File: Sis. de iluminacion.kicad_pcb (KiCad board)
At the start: 2 copper layers, 48 parts, among them J1 Screw_Terminal_01x02, J2 Screw_Terminal_01x04, J3 Screw_Terminal_01x02, J5 Screw_Terminal_01x02, J7 Screw_Terminal_01x02, J9 Screw_Terminal_01x02, K10 Relay_DPDT, K11 Relay_DPDT, K8 Relay_DPDT, K9 Relay_DPDT, Q4 BC547, Q5 BC547, Q6 BC547, Q7 BC547, U1 ESP32_DEVKITC, U10 PC817, U11 PC817, U12 PC817, U13 PC817, U3 L7805

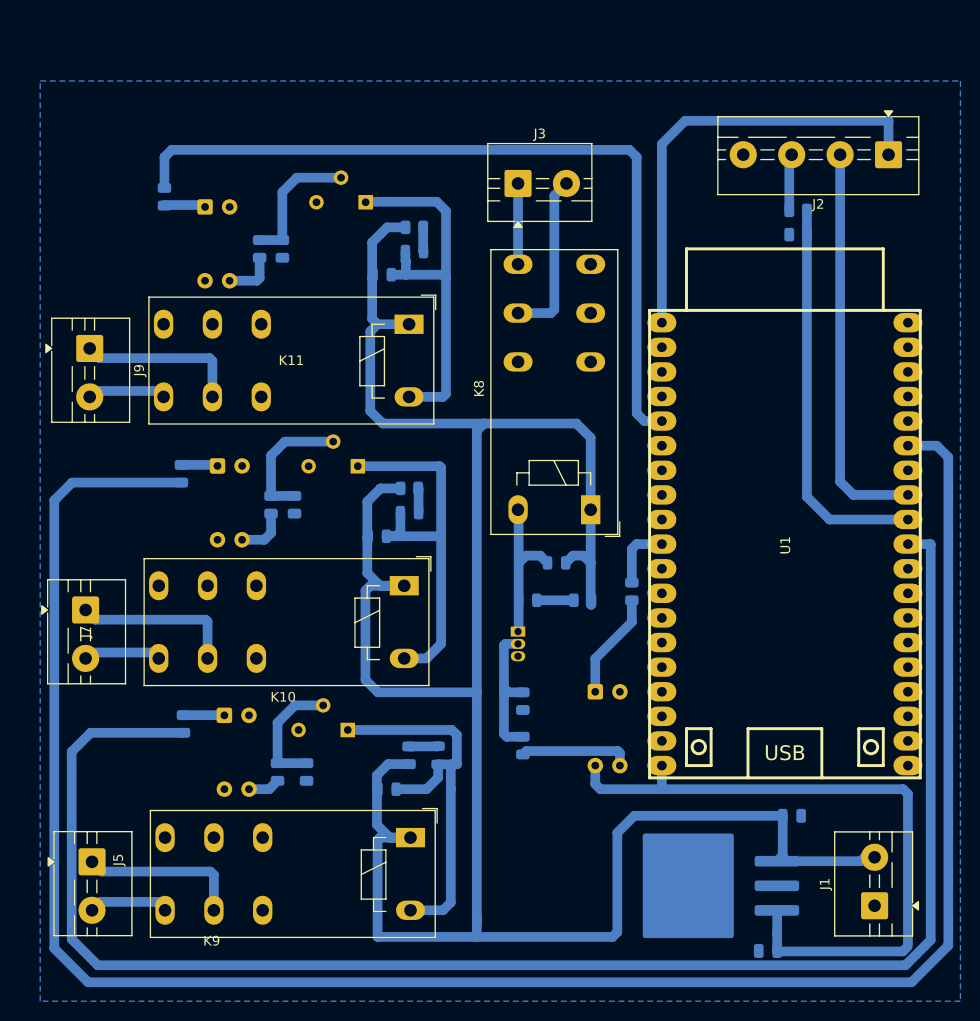
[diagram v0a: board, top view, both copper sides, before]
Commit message: Rele wifi
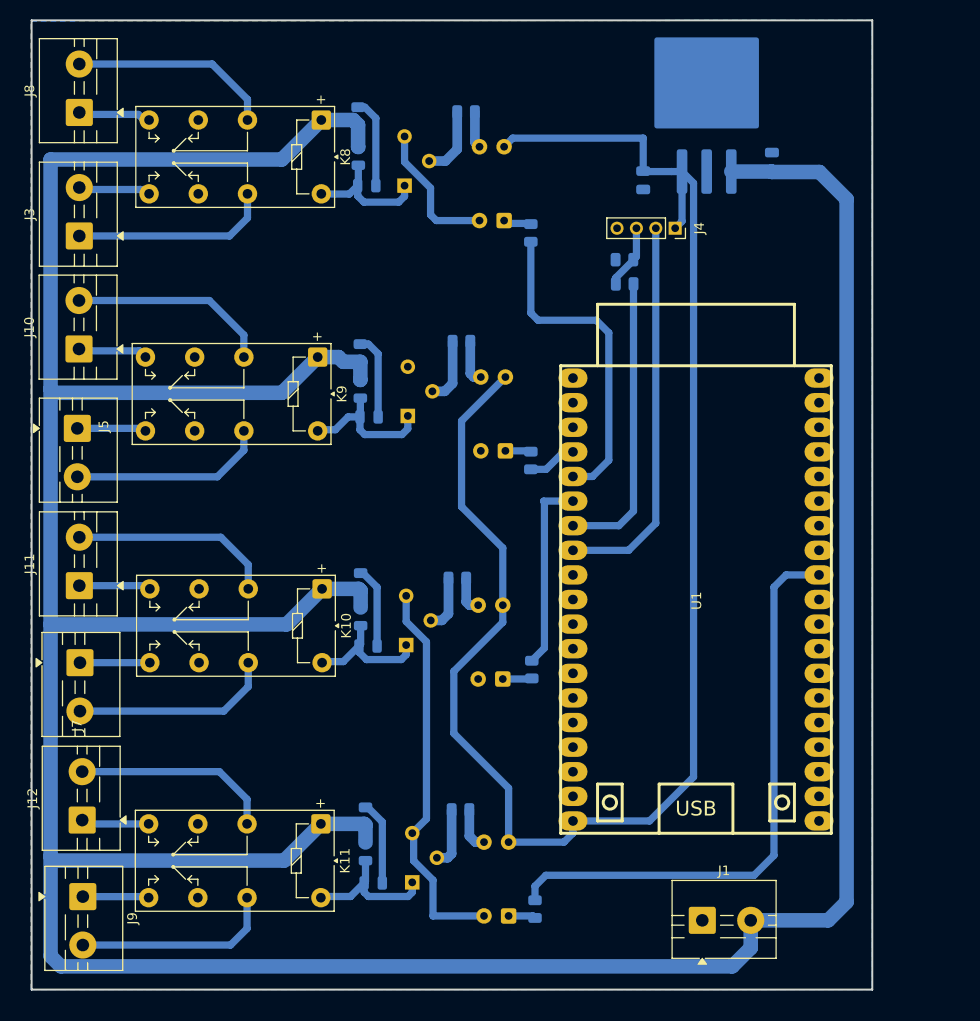
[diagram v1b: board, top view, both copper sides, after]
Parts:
- removed J2: Screw_Terminal_01x04, TerminalBlock:TerminalBlock_MaiXu_MX126-5.0-04P_1x04_P5.00mm
- removed R26, R31, R35, R39: 10K, Resistor_SMD:R_0805_2012Metric
- added J10: Screw_Terminal_01x02, TerminalBlock:TerminalBlock_MaiXu_MX126-5.0-02P_1x02_P5.00mm, F.Cu at (185.0, 74.2)
- added J11: Screw_Terminal_01x02, TerminalBlock:TerminalBlock_MaiXu_MX126-5.0-02P_1x02_P5.00mm, F.Cu at (185.0, 98.6)
- added J12: Screw_Terminal_01x02, TerminalBlock:TerminalBlock_MaiXu_MX126-5.0-02P_1x02_P5.00mm, F.Cu at (185.3, 122.8)
- added J4: Conn_01x04, Connector_PinSocket_2.00mm:PinSocket_1x04_P2.00mm_Vertical, F.Cu at (246.6, 61.7)
- added J8: Screw_Terminal_01x02, TerminalBlock:TerminalBlock_MaiXu_MX126-5.0-02P_1x02_P5.00mm, F.Cu at (185.0, 49.8)
- K10, K11, K8, K9: footprint Relay_THT:Relay_DPDT_Schrack-RT2-FormC_RM5mm -> Relay_THT:Relay_DPDT_Omron_G6A
- Q4: footprint Package_TO_SOT_THT:TO-92_Inline -> Package_TO_SOT_THT:TO-92_Wide
- R24, R28, R32, R36: value 1K -> 220
- moved R36 82.9 mm to (232.1, 132.0)
- moved U3 81.4 mm to (249.8, 48.2), turned to 90 degrees
- moved C2 80.6 mm to (243.2, 56.8), turned to -90 degrees
- moved U13 79.6 mm to (229.4, 132.7), turned to 90 degrees
- moved Q7 70.4 mm to (219.4, 129.2), turned to 90 degrees
- moved C1 67.6 mm to (256.5, 54.8), turned to 90 degrees
- moved R25 65.7 mm to (225.0, 49.7), turned to 180 degrees
- moved D21 65.3 mm to (215.4, 129.3)
- moved R37 61.5 mm to (224.4, 121.8), turned to 180 degrees
- moved R38 61.0 mm to (214.6, 122.4), turned to -90 degrees
- moved D22 59.6 mm to (214.6, 126.1), turned to -90 degrees
- moved J9 56.6 mm to (185.4, 130.7)
- moved R27 55.1 mm to (213.8, 50.1), turned to -90 degrees
- moved K11 52.4 mm to (210.0, 123.2), turned to -90 degrees
- moved K9 50.5 mm to (209.6, 75.0), turned to -90 degrees
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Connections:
- J3 pad 1: LED + -> 5V1
- J3 pad 2: 5V -> LED +
- J5 pad 1: V1 -> NO1
- J5 pad 2: NO1 -> V1
- J7 pad 1: V2 -> NO2
- J7 pad 2: NO2 -> V2
- J9 pad 1: V3 -> NO3
- J9 pad 2: NO3 -> V3
- K10 pad 11: unconnected-(K10-Pad11) -> COM10
- K10 pad 14: unconnected-(K10-Pad14) -> NO10
- K11 pad 11: unconnected-(K11-Pad11) -> COM11
- K11 pad 14: unconnected-(K11-Pad14) -> NO11
- K8 pad 11: unconnected-(K8-Pad11) -> COM
- K8 pad 14: unconnected-(K8-Pad14) -> NO
- K8 pad 21: 5V -> 5V1
- K8 pad 22: NC -> unconnected-(K8-Pad22)
- K9 pad 11: unconnected-(K9-Pad11) -> COM9
- K9 pad 14: unconnected-(K9-Pad14) -> NO9
- R16 pad 1: GIOP18 -> GIOP32
- R16 pad 2: Net-(J2-Pin_3) -> Net-(J4-Pin_3)
- R17 pad 2: GIOP18 -> Net-(J4-Pin_3)
- R24 pad 1: GIOP26 -> GIOP34
- R28 pad 1: GIOP5 -> GIOP39
- R32 pad 1: GIOP21 -> GIOP35
- R36 pad 1: GIOP34 -> GIOP18
- U1 pad 1: 3.3V -> unconnected-(U1-3V3-Pad1)
- U1 pad 10: GIOP26 -> unconnected-(U1-IO26-Pad10)
- U1 pad 29: GIOP5 -> unconnected-(U1-IO5-Pad29)
- U1 pad 33: GIOP21 -> unconnected-(U1-IO21-Pad33)
- U1 pad 4: unconnected-(U1-SVN-Pad4) -> GIOP39
- U1 pad 6: unconnected-(U1-IO35-Pad6) -> GIOP35
- U1 pad 7: unconnected-(U1-IO32-Pad7) -> GIOP32
- U1 pad 8: unconnected-(U1-IO33-Pad8) -> GIOP33
- U11 pad 4: unconnected-(U11-Pad4) -> +5V
- U12 pad 4: unconnected-(U12-Pad4) -> +5V
- U13 pad 4: unconnected-(U13-Pad4) -> +5V
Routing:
- net GIOP21: track 210.5 -> 0.00 mm
- net GIOP5: track 165.8 -> 0.00 mm
- net +12V: track 259.7 -> 398.2 mm
- net +5V: track 70.5 -> 170.3 mm
- net GND: track 0.00 -> 55.2 mm
- net GIOP34: track 81.9 -> 33.8 mm
- net 3.3V: track 46.3 -> 0.00 mm
- net GIOP19: track 41.3 -> 0.00 mm
- net GIOP33: track 0.00 -> 40.2 mm
- net GIOP32: track 0.00 -> 30.3 mm
- net Net-(D19-K): track 40.6 -> 13.8 mm
- net Net-(D17-K): track 41.4 -> 14.9 mm
- net Net-(D21-K): track 39.7 -> 14.7 mm
- net COM10: track 0.00 -> 21.1 mm
- net COM: track 0.00 -> 21.0 mm
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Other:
- board outline added: 86.8 x 100.1 mm
